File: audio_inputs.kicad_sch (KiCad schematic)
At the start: 12 parts, among them J2 AFBR-2624Z, U4 DIR9001PW, Y1 12.288 MHz

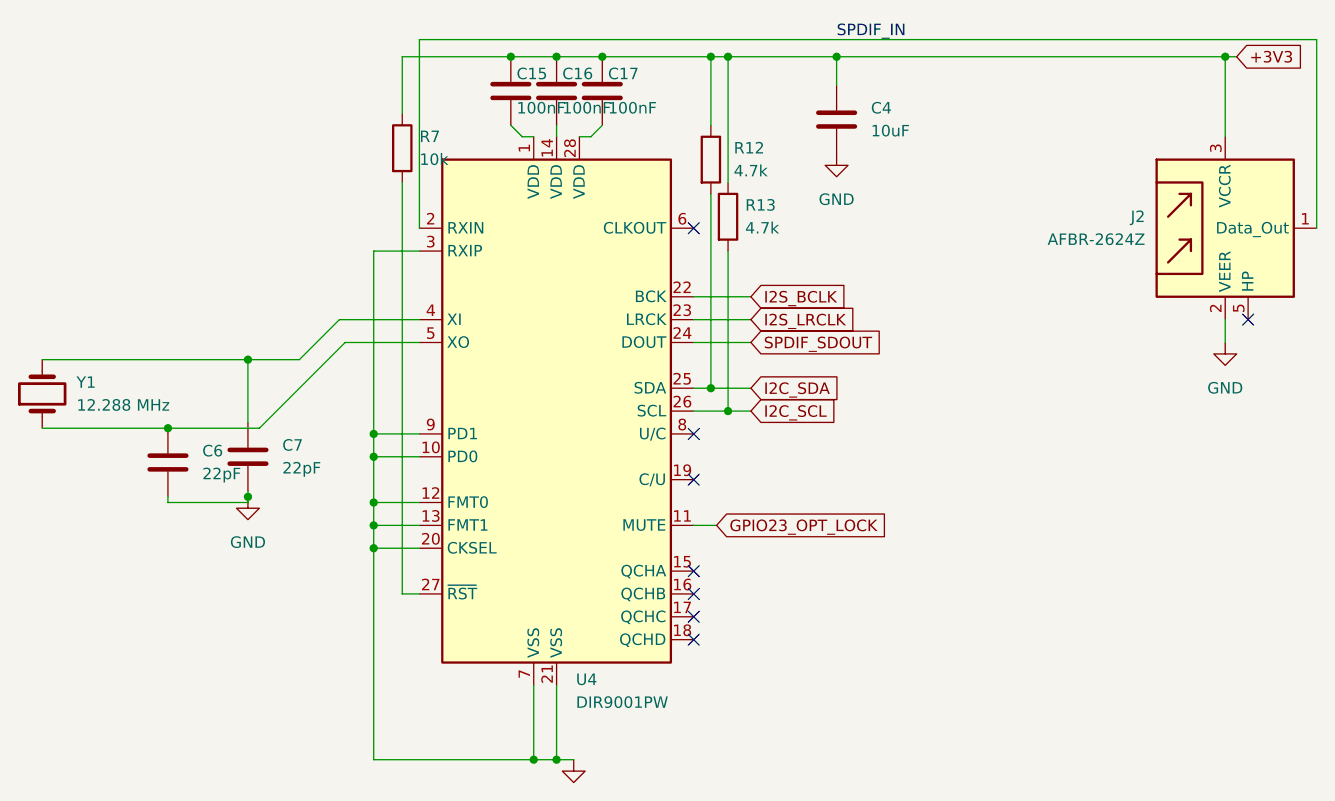
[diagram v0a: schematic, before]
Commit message: visiually cleaned up DIR9000
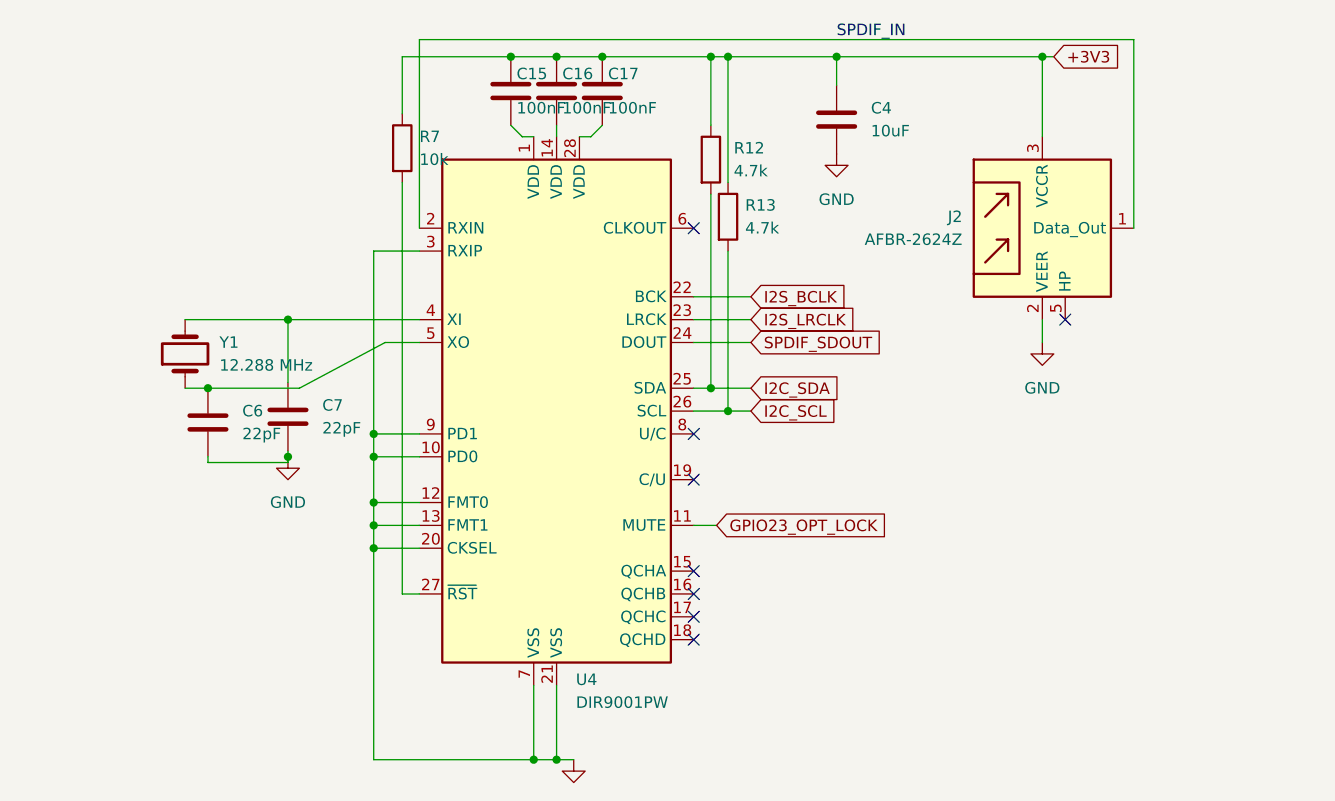
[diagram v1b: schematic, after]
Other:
- moved on the sheet: C6, C7, J2, Y1
